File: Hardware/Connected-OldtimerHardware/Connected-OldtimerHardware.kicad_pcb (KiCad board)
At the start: 2 copper layers, 1 part, among them U1 electron

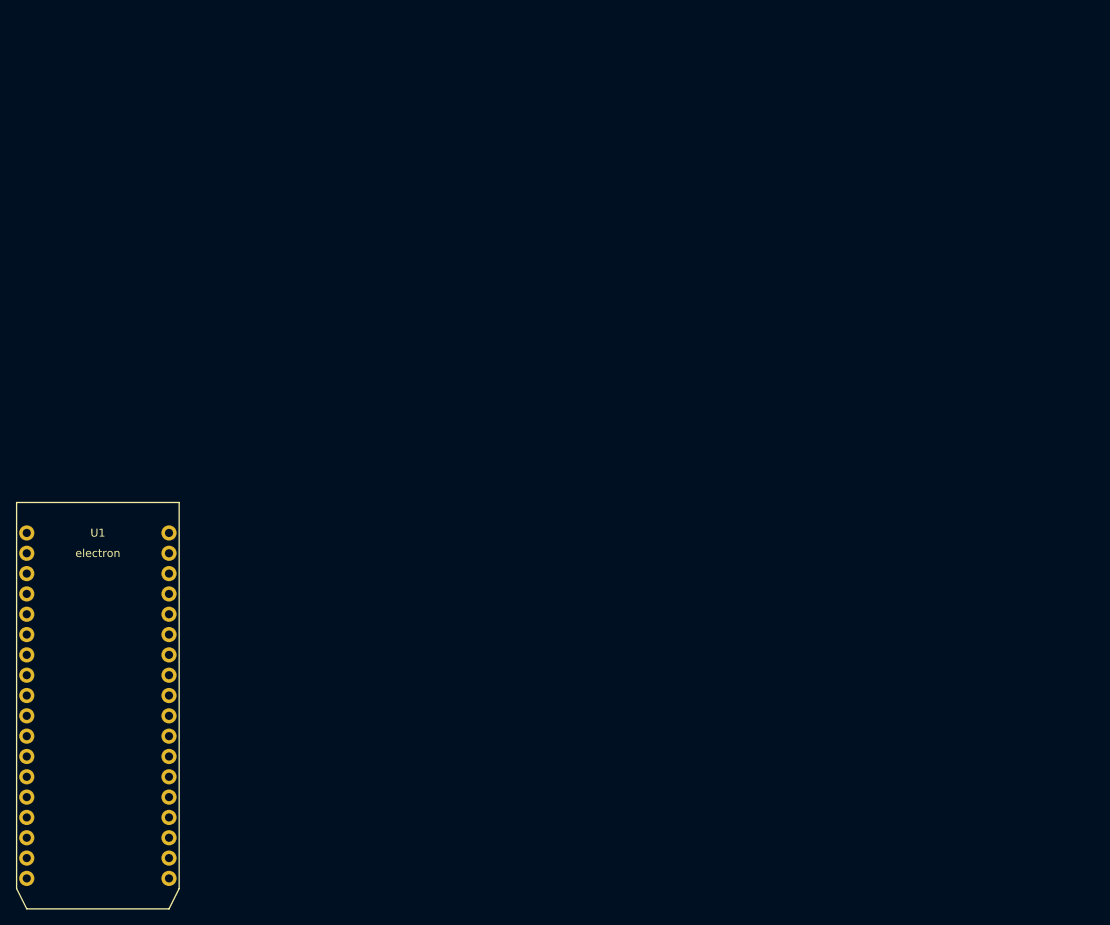
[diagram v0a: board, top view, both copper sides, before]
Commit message: layout v1
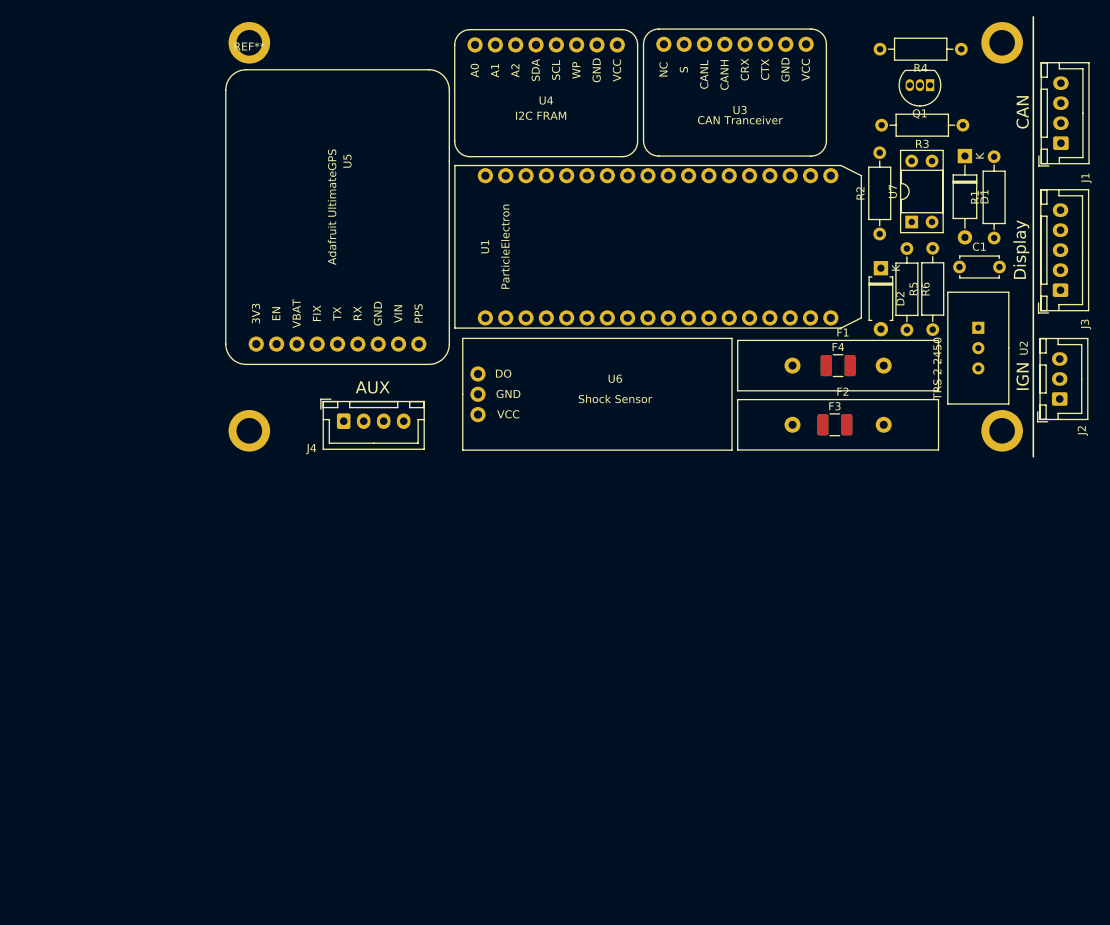
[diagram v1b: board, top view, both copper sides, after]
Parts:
- added C1: 1uF, Capacitor_THT:C_Disc_D4.7mm_W2.5mm_P5.00mm, F.Cu at (185.2, 95.0)
- added D1: DIODE, Diode_THT:D_A-405_P10.16mm_Horizontal, F.Cu at (185.9, 81.2)
- added D2: D_Zener, Diode_THT:D_A-405_P7.62mm_Horizontal, F.Cu at (175.3, 95.2)
- added F1: Polyfuse 2000mA, Fuse:Fuse_Littelfuse-LVR200, F.Cu at (164.3, 107.3)
- added F2: Polyfuse 1000mA, Fuse:Fuse_Littelfuse-LVR200, F.Cu at (164.3, 114.8)
- added F3: Polyfuse SMD 1000mA, Capacitor_SMD:C_1210_3225Metric_Pad1.42x2.65mm_HandSolder, F.Cu at (169.6, 114.8)
- added F4: Polyfuse SMD 2000mA, Capacitor_SMD:C_1210_3225Metric_Pad1.42x2.65mm_HandSolder, F.Cu at (170.0, 107.3)
- added J1: CAN_Bus_Connector, Connector_JST:JST_XH_B04B-XH-A_1x04_P2.50mm_Vertical, F.Cu at (197.8, 79.5)
- added J2: MainConnector, Connector_JST:JST_XH_B03B-XH-A_1x03_P2.50mm_Vertical, F.Cu at (197.7, 111.5)
- added J3: NextionConnector, Connector_JST:JST_XH_B05B-XH-A_1x05_P2.50mm_Vertical, F.Cu at (197.8, 97.9)
- added J4: Conn_01x04, Connector_JST:JST_XH_B04B-XH-A_1x04_P2.50mm_Vertical, F.Cu at (108.2, 114.3)
- added Q1: 2N3906, Package_TO_SOT_THT:TO-92_Inline, F.Cu at (181.5, 72.3)
- added R1: 7.5K, Resistor_THT:R_Axial_DIN0207_L6.3mm_D2.5mm_P10.16mm_Horizontal, F.Cu at (189.5, 91.4)
- added R2: 10K, Resistor_THT:R_Axial_DIN0207_L6.3mm_D2.5mm_P10.16mm_Horizontal, F.Cu at (175.2, 90.9)
- added R3: 47K, Resistor_THT:R_Axial_DIN0207_L6.3mm_D2.5mm_P10.16mm_Horizontal, F.Cu at (185.6, 77.3)
- added R4: 10K, Resistor_THT:R_Axial_DIN0207_L6.3mm_D2.5mm_P10.16mm_Horizontal, F.Cu at (185.4, 67.8)
- added R5: 31K, Resistor_THT:R_Axial_DIN0207_L6.3mm_D2.5mm_P10.16mm_Horizontal, F.Cu at (181.8, 102.8)
- added R6: 4.7K, Resistor_THT:R_Axial_DIN0207_L6.3mm_D2.5mm_P10.16mm_Horizontal, F.Cu at (178.6, 92.7)
- added REF**: NextionMountingHoles, heathsfootprints:NextionMountingHoles, F.Cu at (96.4, 67.0)
- added U2: TSR_2-2450, heathsfootprints:heathsTRS_2_2450, F.Cu at (187.5, 102.6)
- added U3: CANTranceiverModule, heathsfootprints:CAN_Tranceiver_Module, F.Cu at (154.6, 79.3)
- added U4: AdafruitFRAM, heathsfootprints:Adafruit_I2C_FRAM, F.Cu at (131.0, 76.2)
- added U5: AdafruitUltimateGPS, heathsfootprints:AdafruitUltimateGPS, F.Cu at (108.7, 94.5)
- added U6: MotionSensor, heathsfootprints:ShockSensor, F.Cu at (130.7, 110.3)
- added U7: SFH618A-2, Package_DIP:DIP-4_W7.62mm_Socket, F.Cu at (179.2, 89.4)
- U1: value electron -> ParticleElectron
- moved U1 126.3 mm to (172.9, 92.5), turned to 90 degrees
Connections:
- U1 pad 1: (no net) -> 5VDC
- U1 pad 10: (no net) -> Net-(U1-Pad10)
- U1 pad 11: (no net) -> Net-(U1-Pad11)
- U1 pad 12: (no net) -> Net-(U1-Pad12)
- U1 pad 13: (no net) -> Net-(U1-Pad13)
- U1 pad 14: (no net) -> VMON
- U1 pad 15: (no net) -> AUX_1
- U1 pad 16: (no net) -> AUX_2
- U1 pad 17: (no net) -> Net-(U1-Pad17)
- U1 pad 18: (no net) -> Net-(U1-Pad18)
- U1 pad 19: (no net) -> GPS_TX
- U1 pad 2: (no net) -> GND
- U1 pad 20: (no net) -> GPS_RX
- U1 pad 21: (no net) -> Nextion_TX
- U1 pad 22: (no net) -> Nextion_RX
- U1 pad 23: (no net) -> CAN_TX
- U1 pad 24: (no net) -> CAN_RX
- U1 pad 25: (no net) -> FRAM_SDA
- U1 pad 26: (no net) -> FRAM_SCL
- U1 pad 27: (no net) -> Net-(U1-Pad27)
- U1 pad 28: (no net) -> Net-(U1-Pad28)
- U1 pad 29: (no net) -> Net-(U1-Pad29)
- U1 pad 3: (no net) -> TX
- U1 pad 30: (no net) -> Net-(U1-Pad30)
- U1 pad 31: (no net) -> Net-(U1-Pad31)
- U1 pad 32: (no net) -> Net-(U1-Pad32)
- U1 pad 33: (no net) -> GND
- U1 pad 34: (no net) -> VBAT
- U1 pad 35: (no net) -> RESET
- U1 pad 36: (no net) -> 3V3
- U1 pad 4: (no net) -> RX
- U1 pad 5: (no net) -> Shock_Signal
- U1 pad 6: (no net) -> DAC
- U1 pad 7: (no net) -> Net-(U1-Pad7)
- U1 pad 8: (no net) -> Net-(U1-Pad8)
- U1 pad 9: (no net) -> AUX_3
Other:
- board text added: "AUX"
- board text added: "CAN"
- board text added: "Display"
- board text added: "IGN"
